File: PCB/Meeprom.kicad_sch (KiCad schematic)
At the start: 5 parts, among them J1 Molex 78805 socket with 27C25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, U1 28C256 / FM18W08

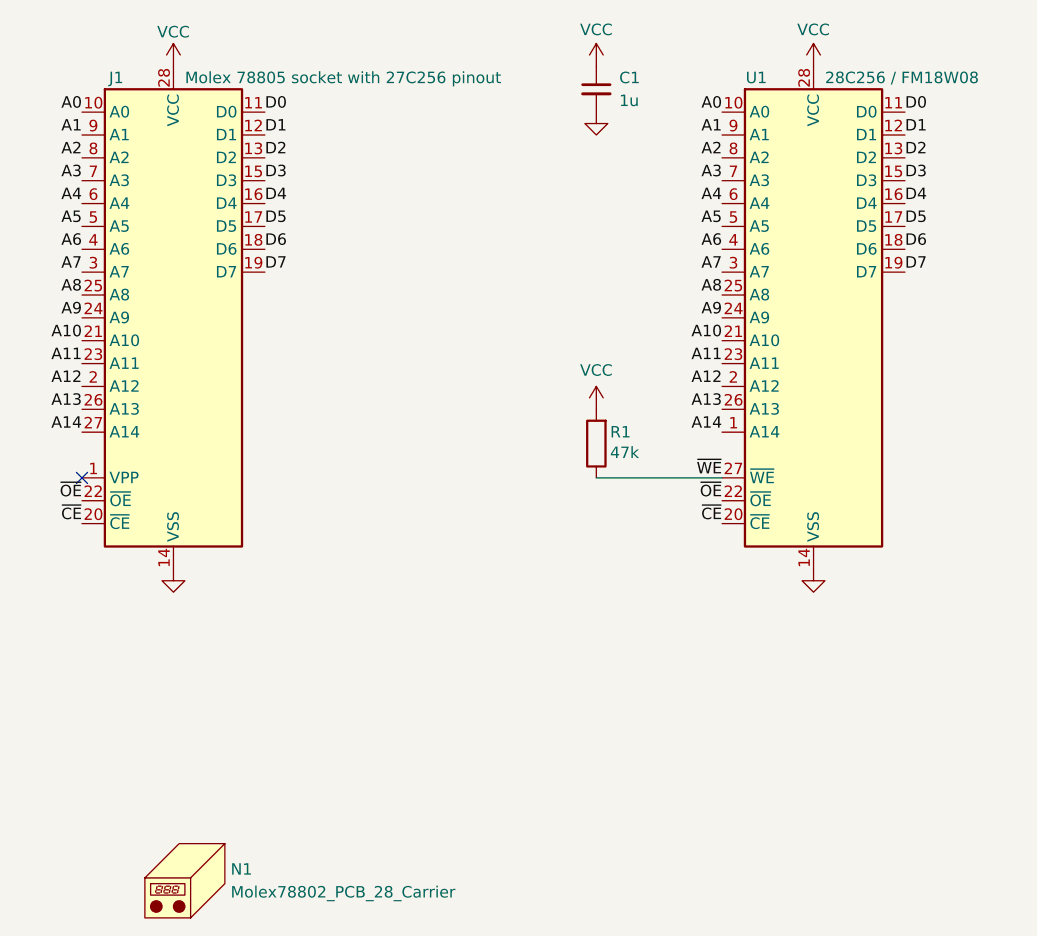
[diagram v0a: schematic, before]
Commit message: bom
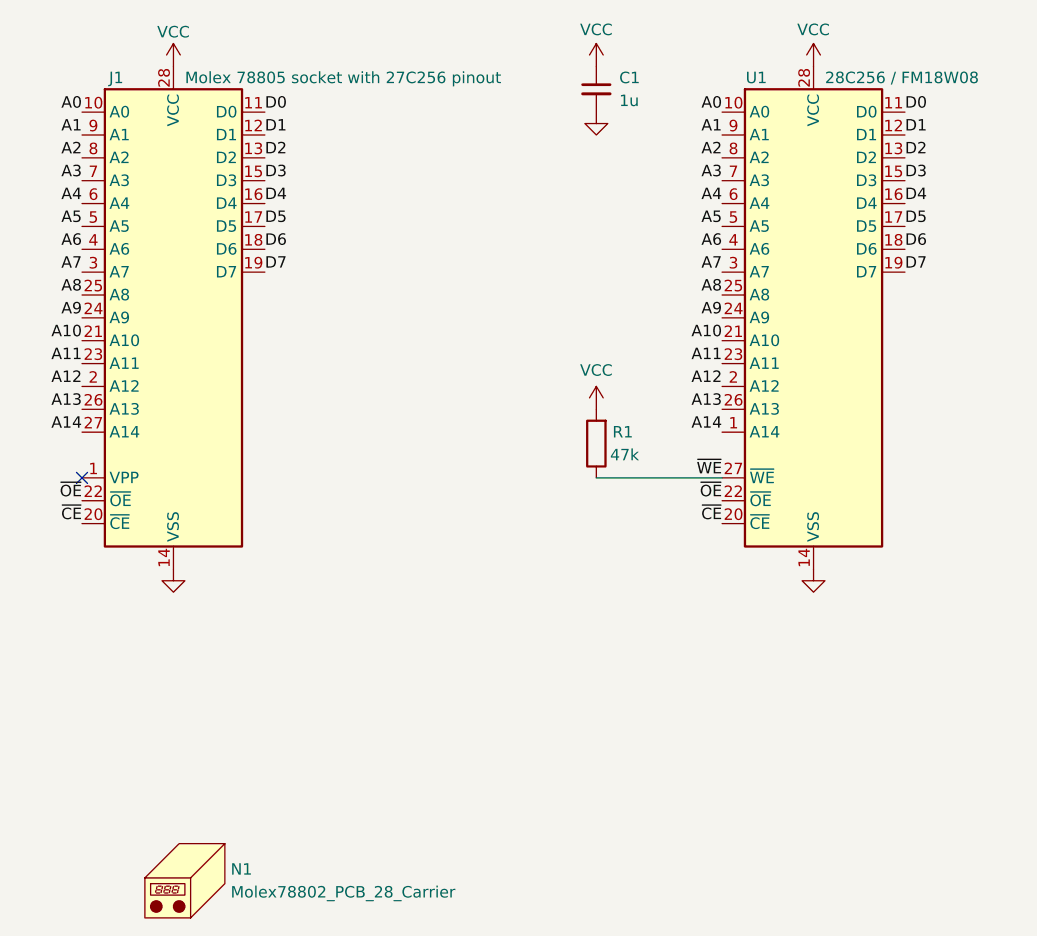
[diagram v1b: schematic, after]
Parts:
- R1: MPN (none) -> CRCW080547K0FKEA
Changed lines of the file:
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@@
 	(title_block
 		(title "Meeprom-28")
-		(date "2022-12-21")
+		(date "2026-02-23")
 		(rev "005")
 		(comment 3 "28C256 to Molex 78805 socket with 27C256 pinout")
@@
 		(dnp no)
 		(property "Reference" "R1"
-			(at 160.274 102.87 0)
+			(at 160.528 102.87 0)
 			(effects
 				(font
@@
 		)
 		(property "Value" "47k"
-			(at 160.274 105.156 0)
+			(at 160.274 105.41 0)
 			(effects
 				(font
@@
 			)
 		)
-		(property "Datasheet" "~"
+		(property "Datasheet" "datasheets/dcrcwe3.pdf"
 			(at 158.75 104.14 0)
 			(effects
@@
 			)
 		)
-		(property "Description" ""
+		(property "Description" "R 47K 1% 0.25W 0805"
+			(at 158.75 93.726 0)
+			(effects
+				(font
+					(size 1.27 1.27)
+				)
+				(hide yes)
+			)
+		)
+		(property "MPN" "CRCW080547K0FKEA"
 			(at 158.75 104.14 0)
 			(effects
@@
 					(size 1.27 1.27)
 				)
+				(hide yes)
 			)
 		)
@@
 		(at 114.3 152.4 0)
 		(unit 1)
-		(exclude_from_sim no)
+		(exclude_from_sim yes)
 		(in_bom no)
 		(on_board yes)
